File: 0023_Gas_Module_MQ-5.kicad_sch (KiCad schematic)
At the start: 11 parts, among them U1 LM393D, U2 MQ-6

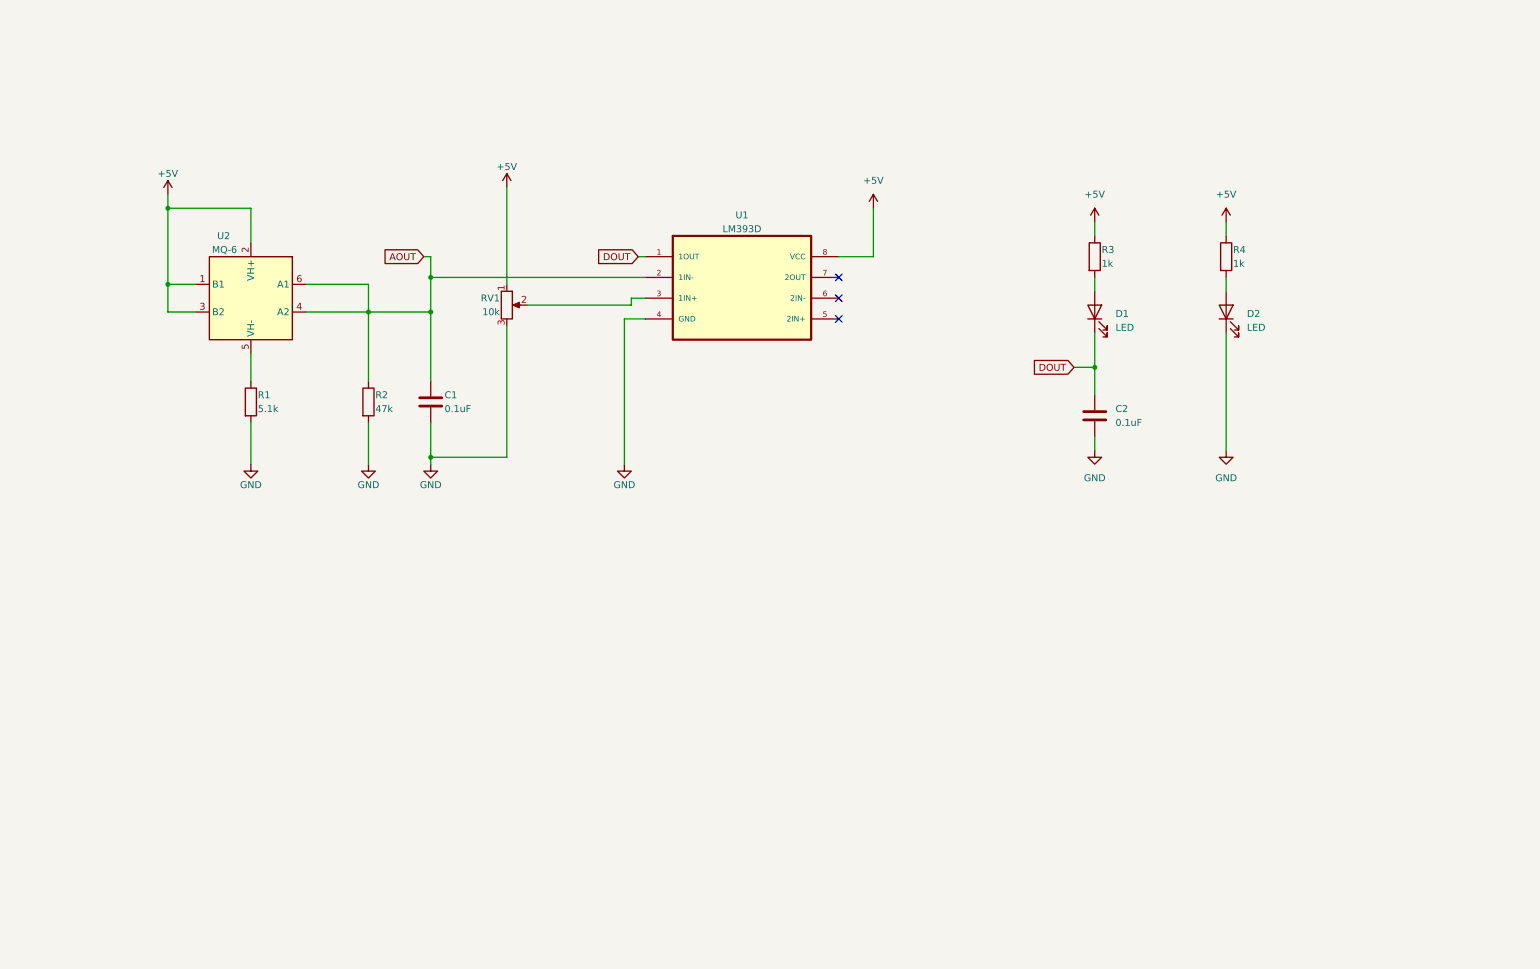
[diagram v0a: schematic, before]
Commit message: Add files via upload
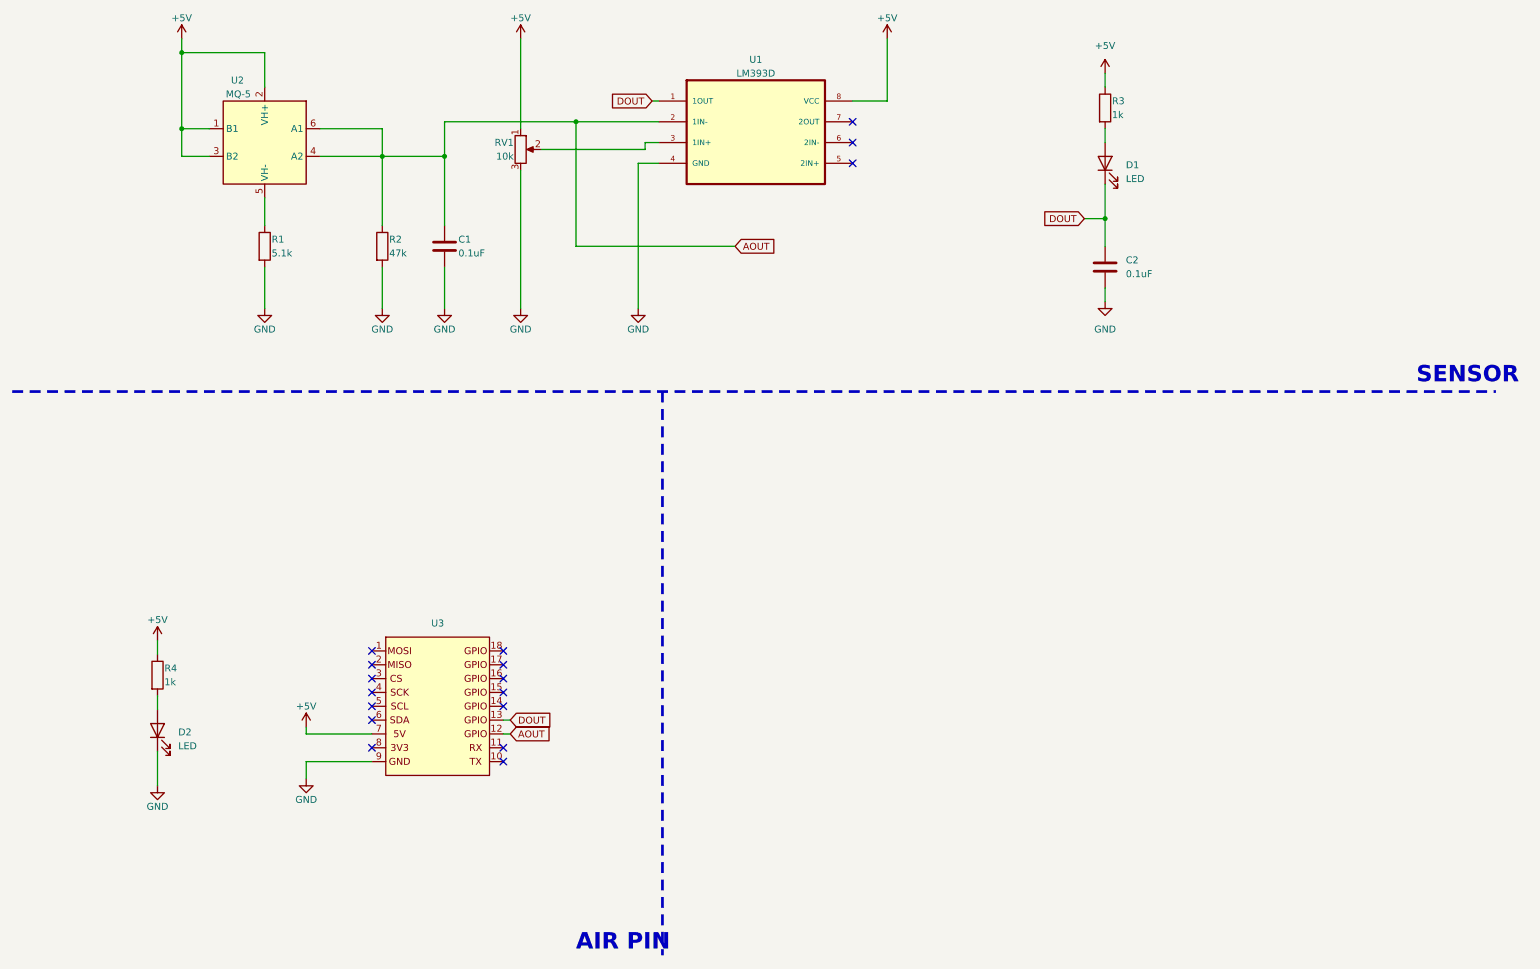
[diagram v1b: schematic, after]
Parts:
- added U3: ~, Moduler_:pin_header, symbol moduler_pin:air
- C1, C2: footprint (none) -> Capacitor_SMD:C_0805_2012Metric
- D1, D2: footprint (none) -> LED_SMD:LED_0805_2012Metric
- R1, R2, R3, R4: footprint (none) -> Resistor_SMD:R_0805_2012Metric
- RV1: footprint (none) -> memin:3362P_1
- U1: footprint SOIC127P599X175-8N -> LM393:SOIC127P599X175-8N
- U2: value MQ-6 -> MQ-5
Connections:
- net +5V: now also U3.7
- net AOUT: now also U3.12
- net DOUT: now also U3.13
- net GND: now also U3.9
- no-connect marks 3 -> 17
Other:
- note added: "AIR PIN"
- note added: "SENSOR"
- moved on the sheet: C1, C2, D1, D2, R1, R2, R3, R4, RV1, U1, U2
